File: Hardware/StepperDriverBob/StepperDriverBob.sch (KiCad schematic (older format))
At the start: 26 parts, among them J1 CONN_01X11, P1 CONN_01X02, P2 CONN_01X04, U1 DRV8825

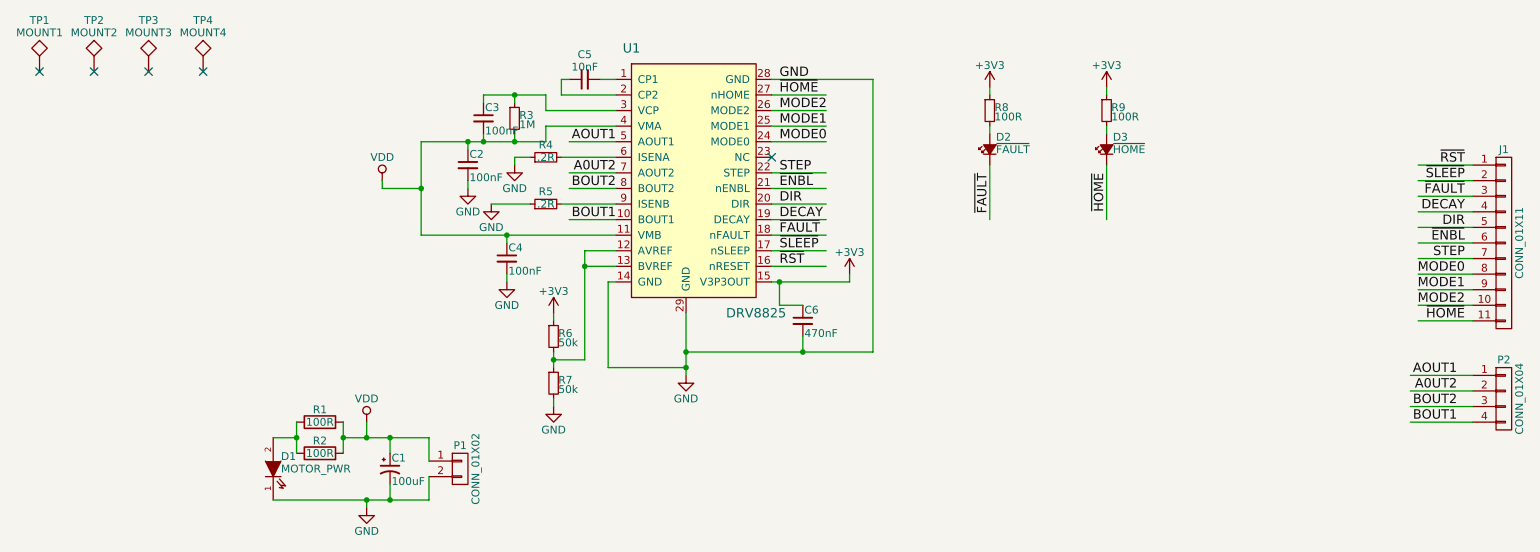
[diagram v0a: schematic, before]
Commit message: I'm not entirely sure
Idk
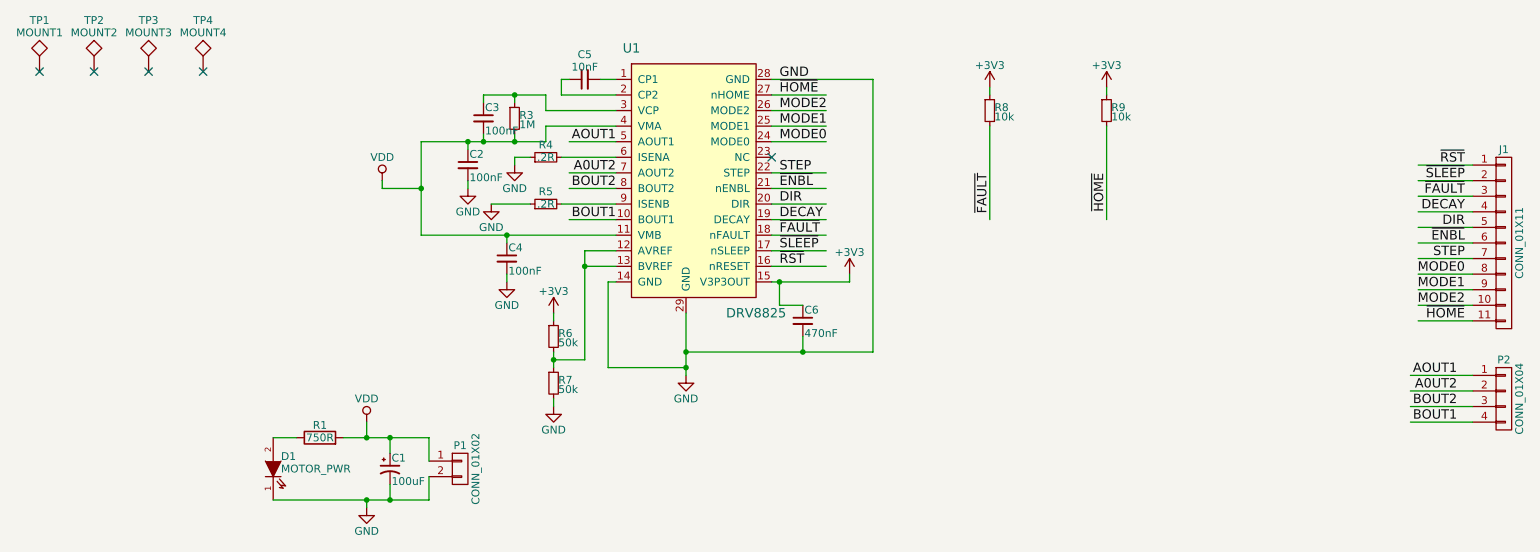
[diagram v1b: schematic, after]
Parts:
- removed D2: ~FAULT~, LEDs:LED_0603, symbol Led_Small
- removed D3: ~HOME~, LEDs:LED_0603, symbol Led_Small
- removed R2: 100R, Resistors_SMD:R_0603, symbol R
- C1: footprint Capacitors_SMD:CP_Elec_5x5.3 -> Capacitors_SMD:CP_Elec_10x10
- R1: value 100R -> 750R
- R8, R9: value 100R -> 10k
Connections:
- wire segments 93 -> 89
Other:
- moved on the sheet: R1
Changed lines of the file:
@@
 F 0 "C1" H 3510 5220 50  0000 L CNN
 F 1 "100uF" H 3510 5070 50  0000 L CNN
-F 2 "Capacitors_SMD:CP_Elec_5x5.3" H 3500 5150 50  0001 C CNN
+F 2 "Capacitors_SMD:CP_Elec_10x10" H 3500 5150 50  0001 C CNN
 F 3 "" H 3500 5150 50  0000 C CNN
 	1    3500 5150
@@
 	1    4250 3800
 	1    0    0    -1
-$EndComp
-$Comp
-L R R2
-U 1 1 58CBDE1A
-P 3050 5050
-F 0 "R2" V 3130 5050 50  0000 C CNN
-F 1 "100R" V 3050 5050 50  0000 C CNN
-F 2 "Resistors_SMD:R_0603" V 2980 5050 50  0001 C CNN
-F 3 "" H 3050 5050 50  0000 C CNN
-	1    3050 5050
-	0    -1   -1   0
 $EndComp
 $Comp
@@
 $EndComp
 $Comp
-L Led_Small D2
-U 1 1 58CCCD00
-P 7350 3100
-F 0 "D2" V 7430 3060 50  0000 R CNN
-F 1 "~FAULT~" V 7350 3060 50  0000 R CNN
-F 2 "LEDs:LED_0603" V 7350 3100 50  0001 C CNN
-F 3 "" V 7350 3100 50  0000 C CNN
-	1    7350 3100
-	0    -1   -1   0
-$EndComp
-$Comp
-L R_Small R8
-U 1 1 58CCCE55
-P 7350 2850
-F 0 "R8" H 7380 2870 50  0000 L CNN
-F 1 "100R" H 7380 2810 50  0000 L CNN
-F 2 "Resistors_SMD:R_0603" H 7350 2850 50  0001 C CNN
-F 3 "" H 7350 2850 50  0000 C CNN
-	1    7350 2850
-	1    0    0    -1
-$EndComp
-$Comp
 L R_Small R9
 U 1 1 58CD2500
 P 8100 2850
 F 0 "R9" H 8130 2870 50  0000 L CNN
-F 1 "100R" H 8130 2810 50  0000 L CNN
+F 1 "10k" H 8130 2810 50  0000 L CNN
 F 2 "Resistors_SMD:R_0603" H 8100 2850 50  0001 C CNN
 F 3 "" H 8100 2850 50  0000 C CNN
 	1    8100 2850
 	1    0    0    -1
-$EndComp
-$Comp
-L Led_Small D3
-U 1 1 58CD3415
-P 8100 3100
-F 0 "D3" V 8180 3060 50  0000 R CNN
-F 1 "~HOME~" V 8100 3060 50  0000 R CNN
-F 2 "LEDs:LED_0603" V 8100 3100 50  0001 C CNN
-F 3 "" V 8100 3100 50  0000 C CNN
-	1    8100 3100
-	0    -1   -1   0
 $EndComp
 $Comp
@@
 	7350 2750 7350 2700
 Wire Wire Line
-	7350 3000 7350 2950
+	7350 2950 7350 3550
 Wire Wire Line
 	8100 2750 8100 2700
 Wire Wire Line
-	8100 2950 8100 3000
+	8100 2950 8100 3550
 Wire Wire Line
 	10100 3300 10450 3300
@@
 Wire Wire Line
 	10050 4650 10450 4650
-Wire Wire Line
-	7350 3200 7350 3550
-Wire Wire Line
-	8100 3200 8100 3550
 Wire Wire Line
 	3450 3300 3450 3350
@@
 L R R1
 U 1 1 5906D58F
-P 3050 4850
-F 0 "R1" V 3130 4850 50  0000 C CNN
-F 1 "100R" V 3050 4850 50  0000 C CNN
-F 2 "Resistors_SMD:R_0603" V 2980 4850 50  0001 C CNN
-F 3 "" H 3050 4850 50  0000 C CNN
-	1    3050 4850
+P 3050 4950
+F 0 "R1" V 3130 4950 50  0000 C CNN
+F 1 "750R" V 3050 4950 50  0000 C CNN
+F 2 "Resistors_SMD:R_0603" V 2980 4950 50  0001 C CNN
+F 3 "" H 3050 4950 50  0000 C CNN
+	1    3050 4950
 	0    -1   -1   0
 $EndComp
-Wire Wire Line
-	3200 4850 3200 5050
-Connection ~ 3200 4950
-Wire Wire Line
-	2900 4850 2900 5050
-Connection ~ 2900 4950
+$Comp
+L R_Small R8
+U 1 1 58CCCE55
+P 7350 2850
+F 0 "R8" H 7380 2870 50  0000 L CNN
+F 1 "10k" H 7380 2810 50  0000 L CNN
+F 2 "Resistors_SMD:R_0603" H 7350 2850 50  0001 C CNN
+F 3 "" H 7350 2850 50  0000 C CNN
+	1    7350 2850
+	1    0    0    -1
+$EndComp
 $EndSCHEMATC
